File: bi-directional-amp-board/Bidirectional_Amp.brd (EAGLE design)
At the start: 78.5 x 52 mm, 134 parts, among them J1 73415-2061, J10 73415-2061, J11 73415-2061, J12 73415-2061, J2 73415-2061, J4 73415-2061, J5 73415-2061, J6 73415-2061, J7 73415-2061, J8 73415-2061, U1 LTC5536, U10 NC7S32M5X, U11 SN74LV1T34DBVR, U2 LTC6994-1, U3 LTC6994-1, U4 QPC1022, U5 NC7S04M5, U6 TQP9111, U7 TQP3M9035, U8 QPC1022, U9 LTC3428EDDPBF

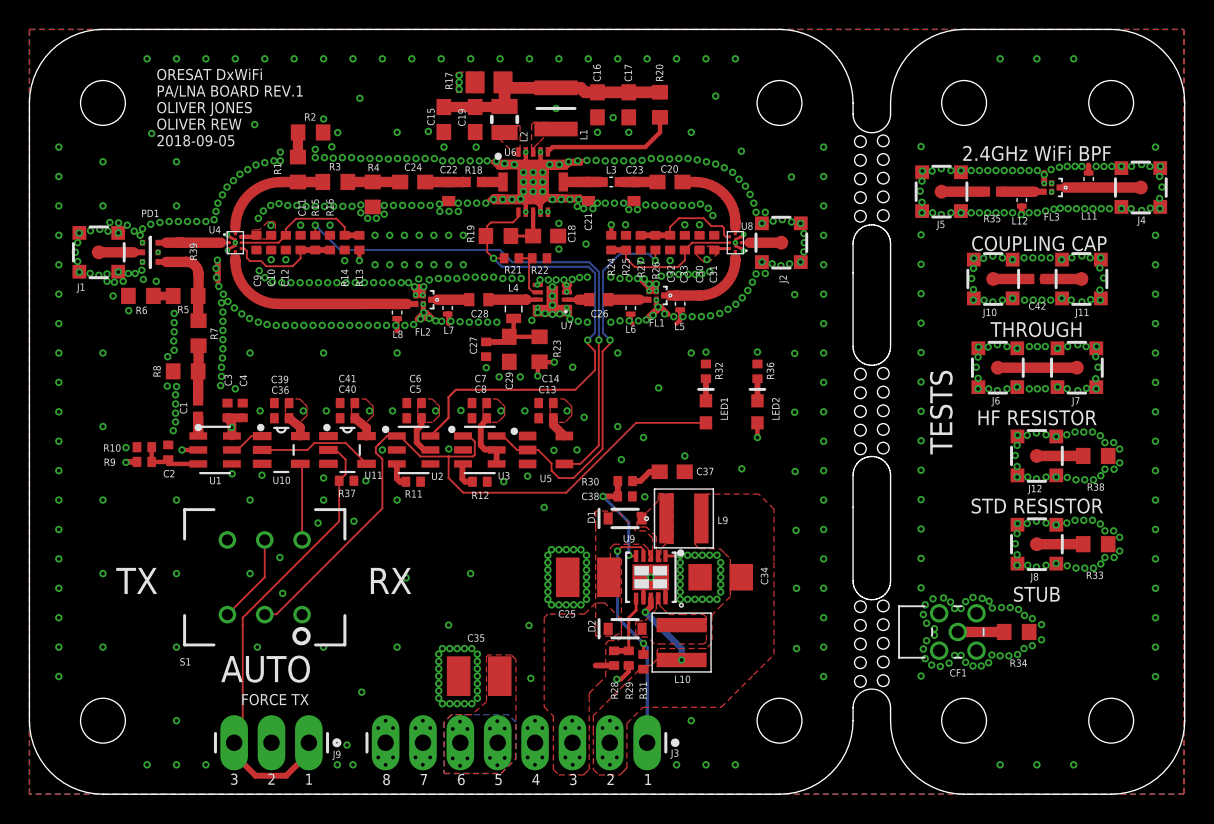
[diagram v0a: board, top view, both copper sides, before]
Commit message: changes from design review
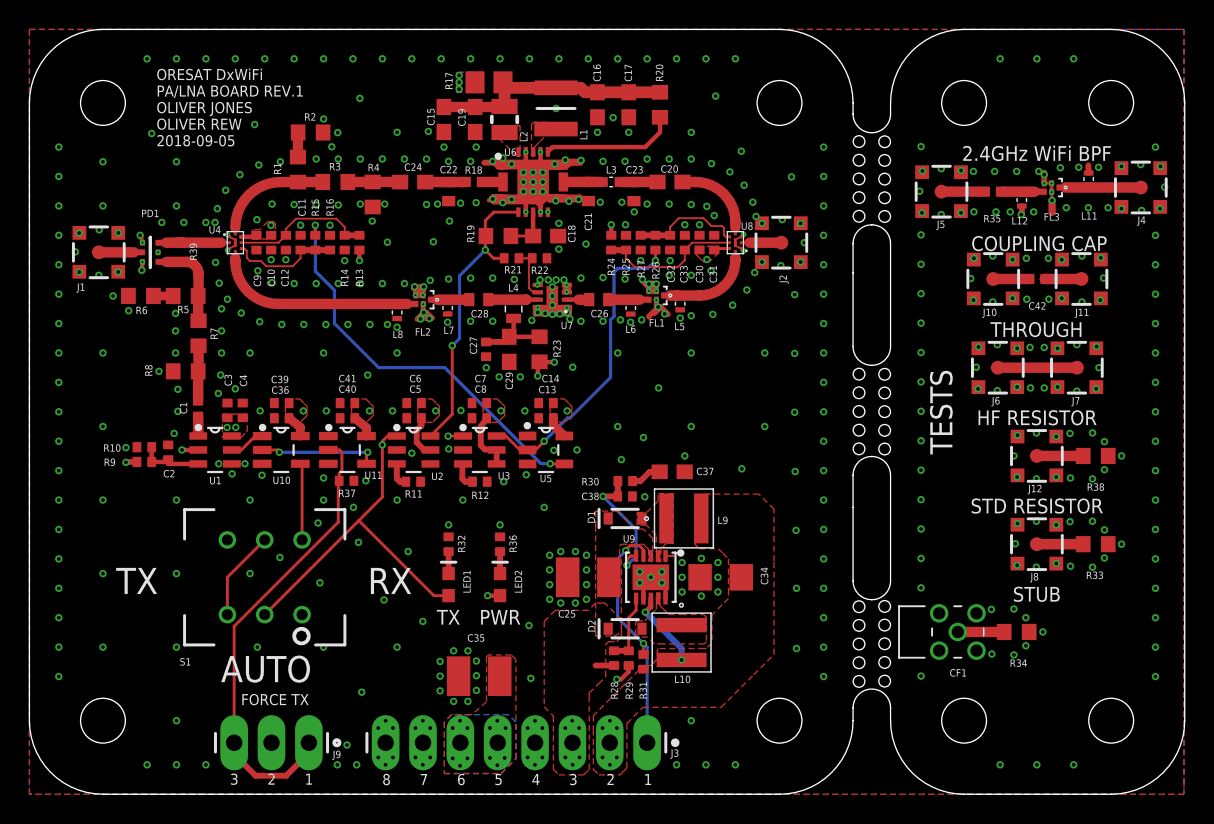
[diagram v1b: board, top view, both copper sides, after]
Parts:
- moved LED1 21.1 mm to (28.5, 14.2)
- moved LED2 21.1 mm to (32.0, 14.2)
- moved R32 21.1 mm to (28.5, 17.0)
- moved R36 21.1 mm to (32.0, 17.0)
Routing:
- net N$10: track 46.3 -> 30.2 mm, vias 0 -> 2
- net PA_ON_LNA_OFF: track 34.1 -> 20.2 mm
- net N$18: track 35.9 -> 27.5 mm
- net TX_RX_CTL: track 27.0 -> 21.3 mm
- net +5V: track 21.7 -> 19.0 mm, vias 23 -> 24
- net VC1: track 7.39 -> 9.13 mm
- net N$3: track 2.45 -> 2.97 mm
- net SHDN1: track 17.3 -> 16.8 mm
- net FORCE_BRDCST_+5V: track 7.87 -> 8.05 mm, vias 0 -> 2
- net GND: track 86.3 -> 86.2 mm, vias 895 -> 566
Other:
- outline, holes or cut-outs redrawn
- board text added: "PWR"
